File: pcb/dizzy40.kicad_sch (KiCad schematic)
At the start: 102 parts, among them U1 ATmega32U2-A, U2 SRV05-4, X1 Crystal_GND24_Small

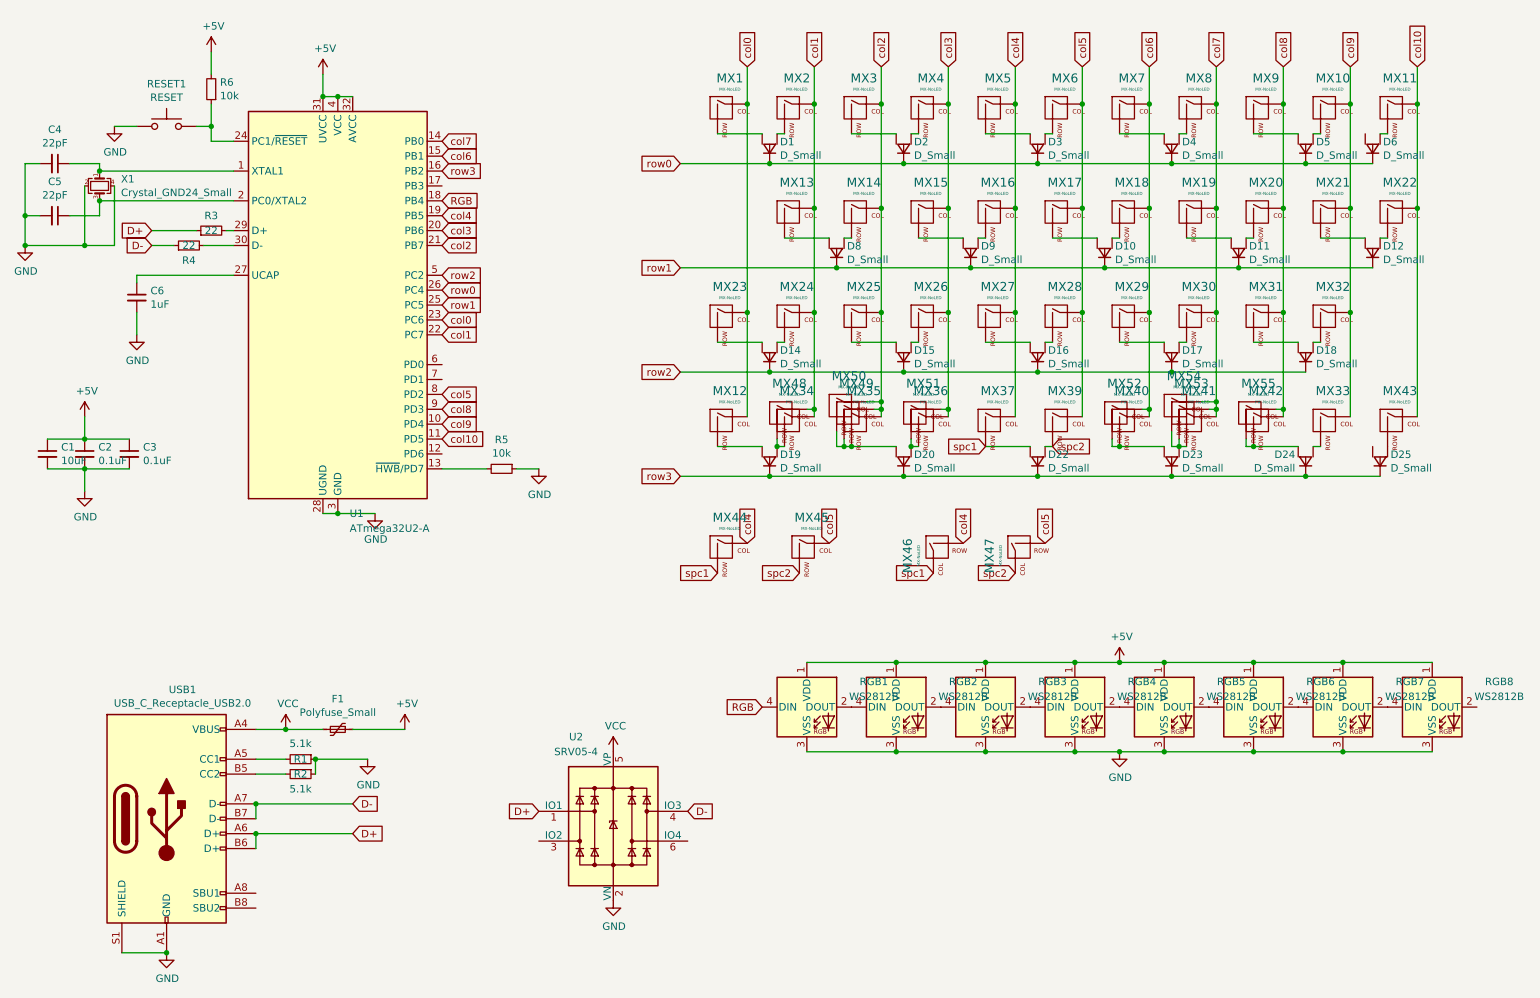
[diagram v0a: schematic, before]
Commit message: outline for updated project
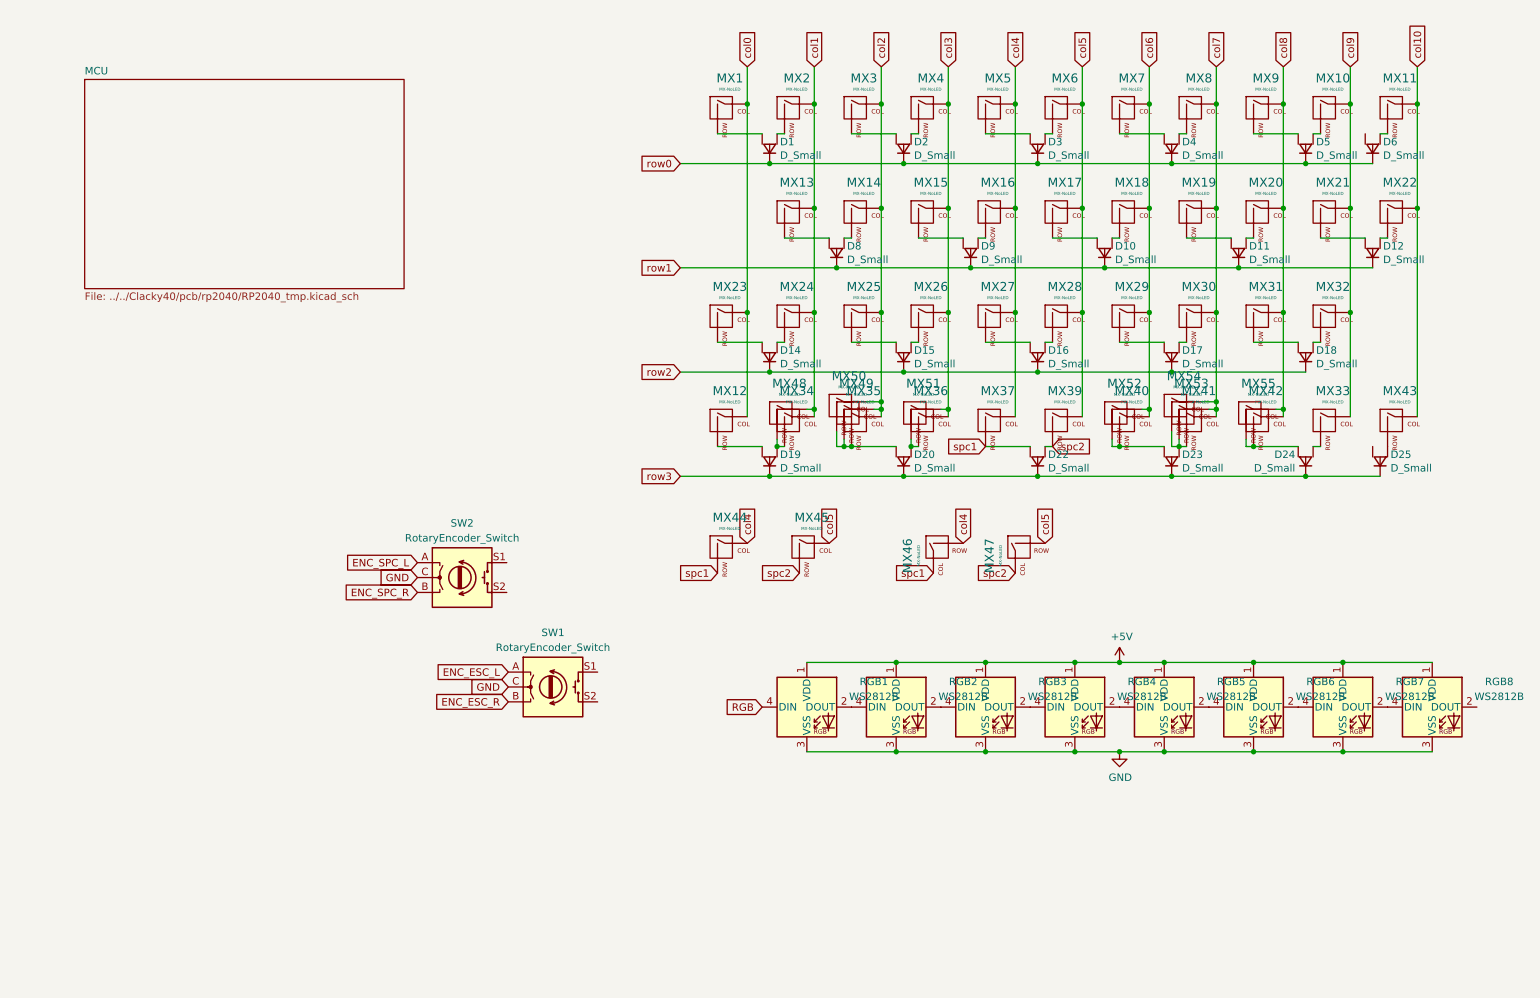
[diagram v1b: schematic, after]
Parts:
- removed C1: 10uF, Capacitor_SMD:C_0805_2012Metric, symbol Device:C_Small
- removed C2, C3: 0.1uF, Capacitor_SMD:C_0805_2012Metric, symbol Device:C_Small
- removed C4, C5: 22pF, Capacitor_SMD:C_0805_2012Metric, symbol Device:C_Small
- removed C6: 1uF, Capacitor_SMD:C_0805_2012Metric, symbol Device:C_Small
- removed F1: Polyfuse_Small, Fuse:Fuse_1206_3216Metric, symbol Device:Polyfuse_Small
- removed R1, R2: 5.1k, Resistor_SMD:R_0805_2012Metric, symbol Device:R_Small
- removed R3, R4: 22, Resistor_SMD:R_0805_2012Metric, symbol Device:R_Small
- removed R5, R6: 10k, Resistor_SMD:R_0805_2012Metric, symbol Device:R_Small
- removed RESET1: RESET, Connector_PinHeader_2.54mm:PinHeader_1x02_P2.54mm_Vertical, symbol Switch:SW_Push
- removed U1: ATmega32U2-A, Package_QFP:TQFP-32_7x7mm_P0.8mm, symbol MCU_Microchip_ATmega:ATmega32U2-A
- removed U2: SRV05-4, Package_TO_SOT_SMD:SOT-23-6, symbol Power_Protection:SRV05-4
- removed USB1: USB_C_Receptacle_USB2.0, Connector_USB:USB_C_Receptacle_HRO_TYPE-C-31-M-12, symbol Connector:USB_C_Receptacle_USB2.0
- removed X1: Crystal_GND24_Small, Crystal:Crystal_SMD_3225-4Pin_3.2x2.5mm, symbol Device:Crystal_GND24_Small
- added SW1, SW2: RotaryEncoder_Switch, symbol Device:RotaryEncoder_Switch
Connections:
- net GND: now also SW1.C, SW2.C
- new net ENC_ESC_L: SW1.A
- new net ENC_ESC_R: SW1.B
- new net ENC_SPC_L: SW2.A
- new net ENC_SPC_R: SW2.B
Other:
- added sheet MCU (../../Clacky40/pcb/rp2040/RP2040_tmp.kicad_sch)
